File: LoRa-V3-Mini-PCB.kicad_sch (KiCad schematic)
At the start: 23 parts, among them Q1 SI2367DS-T1-GE3, SW1 434331045822, SW2 434331045816, U1 114993121, U2 BR24G1MFVT, U3 SHT40, U4 TSL25911

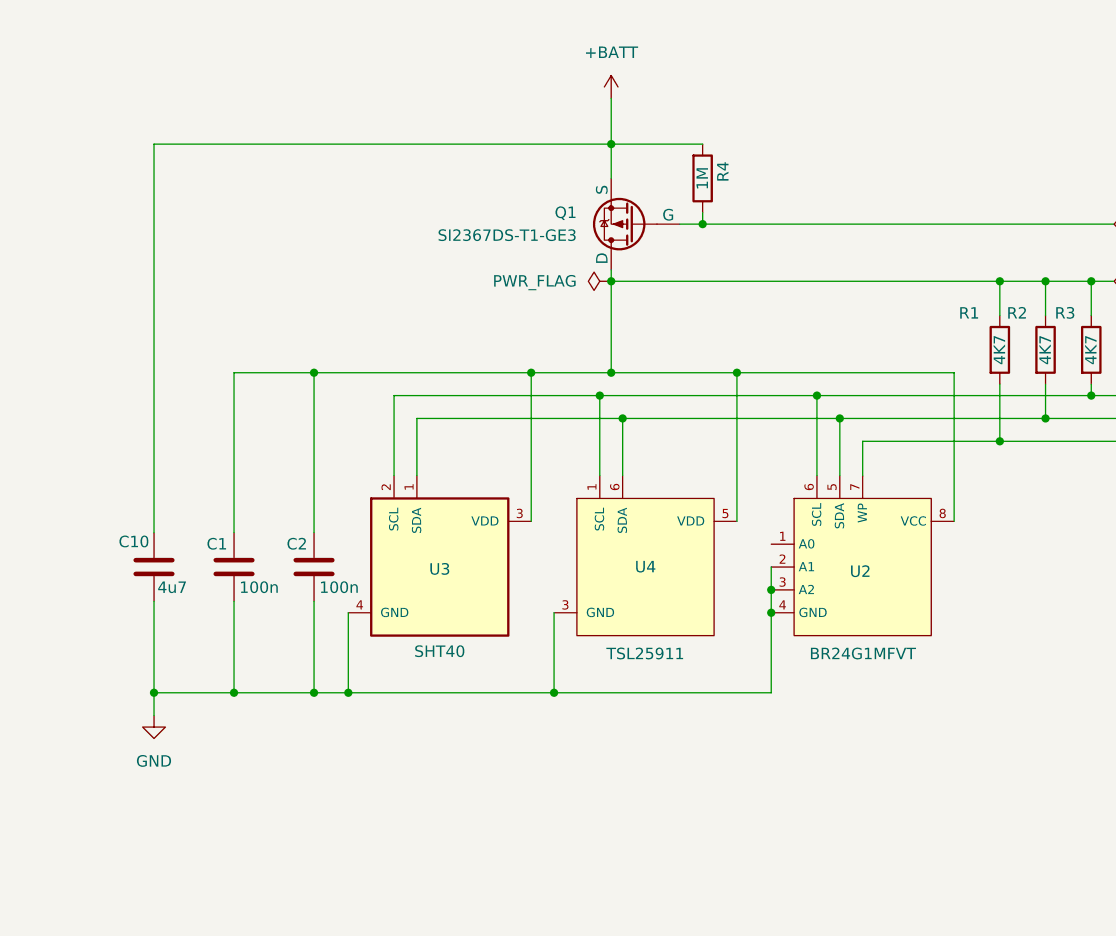
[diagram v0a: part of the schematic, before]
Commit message: finishing touch to layout
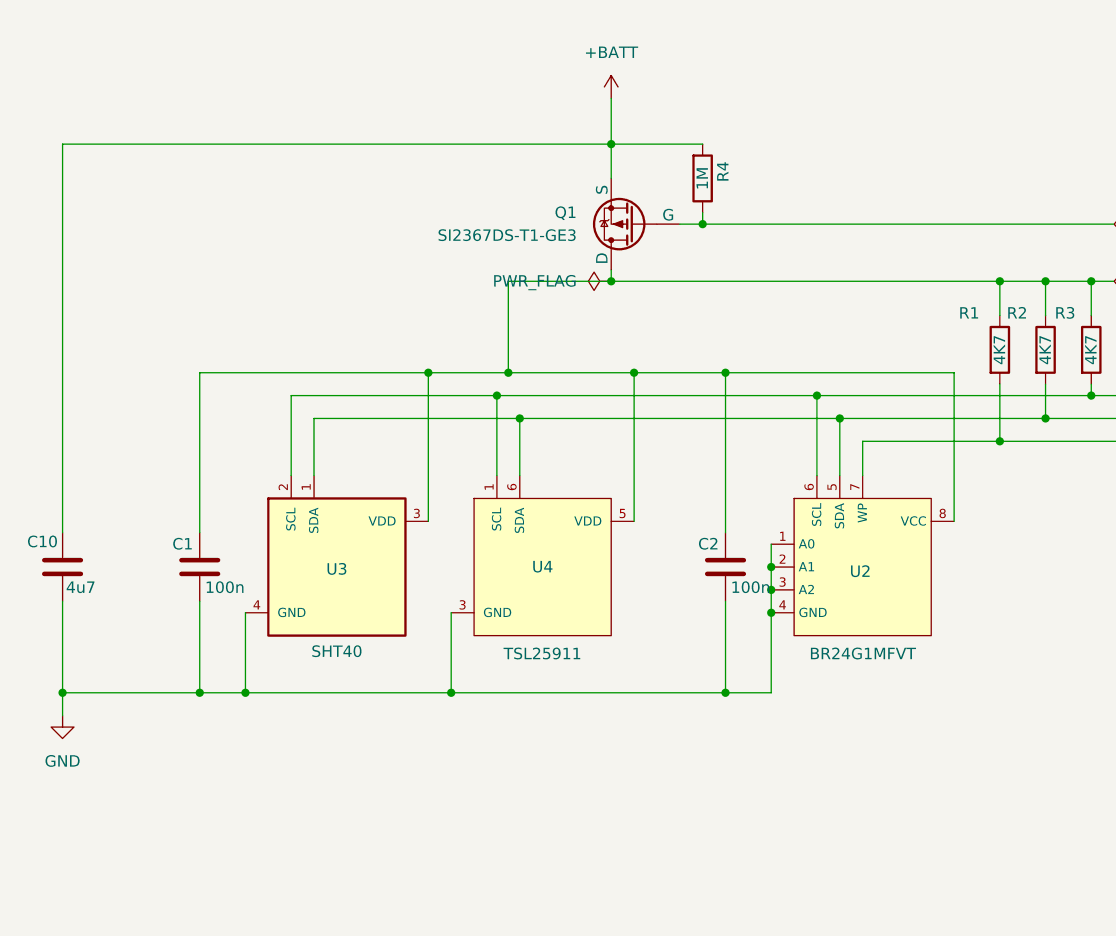
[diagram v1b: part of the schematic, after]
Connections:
- net GND: now also U2.1 (A0)
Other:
- moved on the sheet: C1, C10, C2, U3, U4
